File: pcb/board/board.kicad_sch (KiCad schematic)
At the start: 20 parts, among them J1 USB_C_Receptacle_USB2.0, J3 Micro_SD_Card_Det, J4 Conn_01x05_Male, J6 Conn_02x02_Top_Bottom

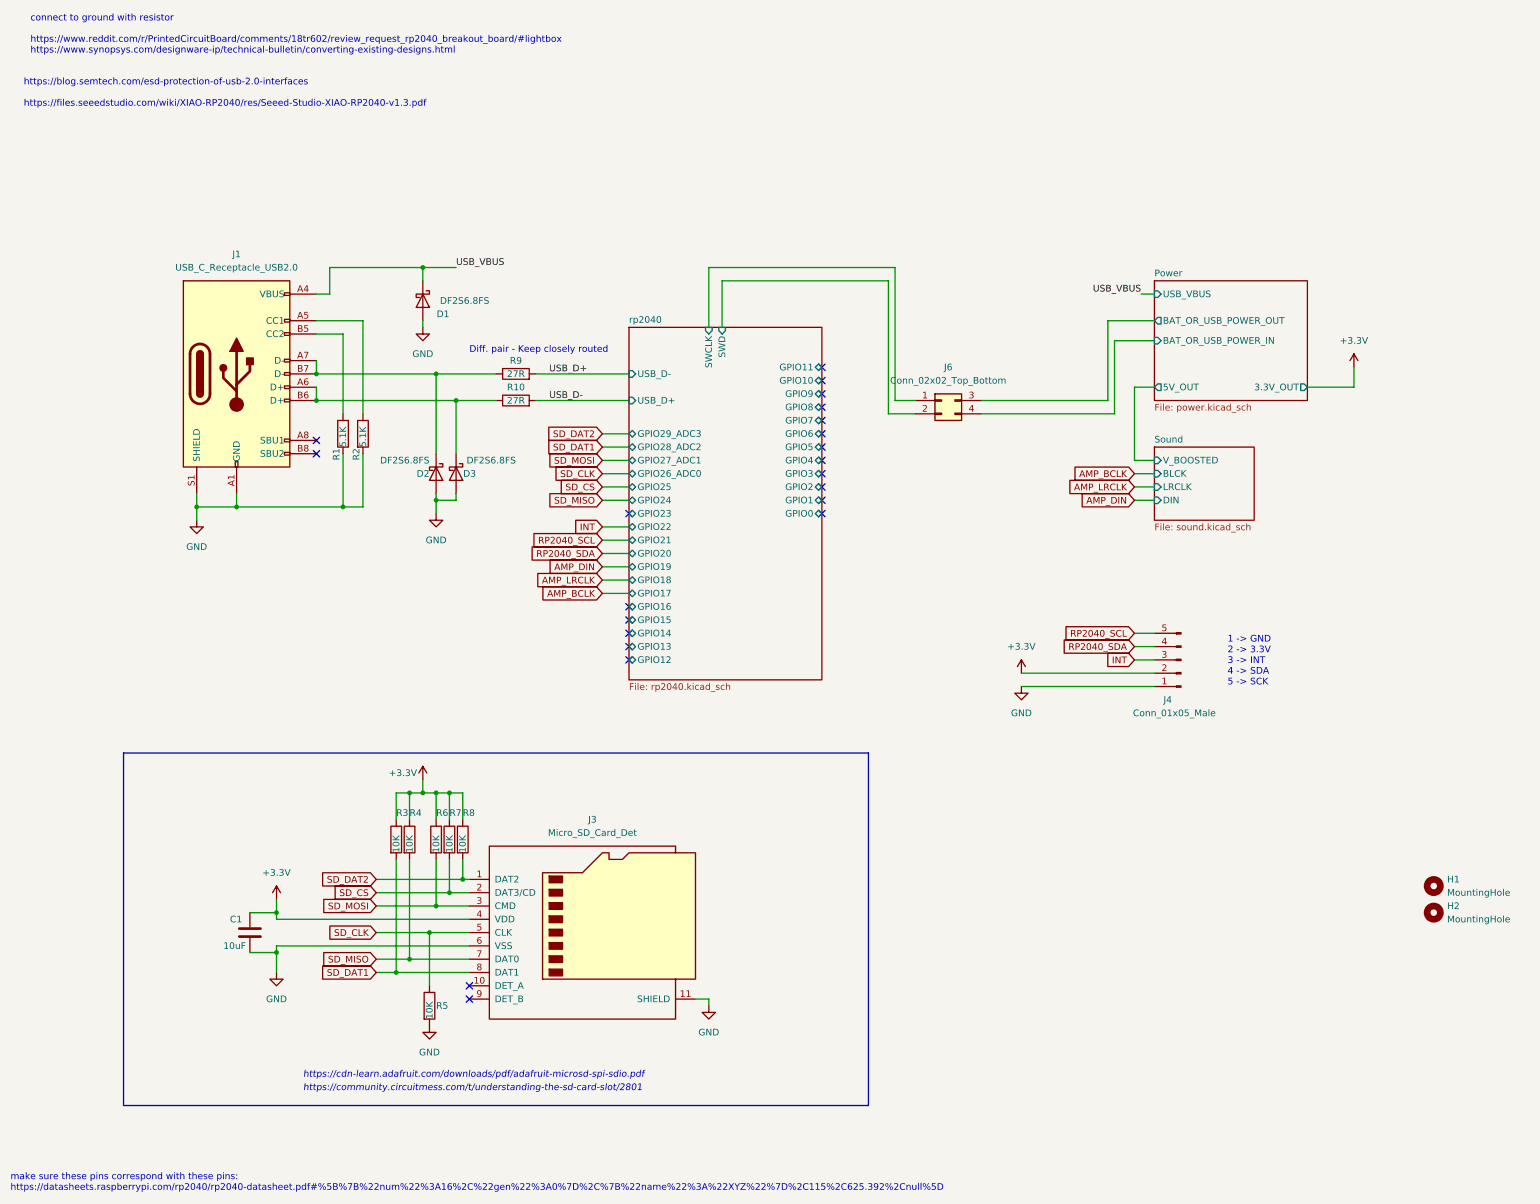
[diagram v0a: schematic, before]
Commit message: Update readme and pcb
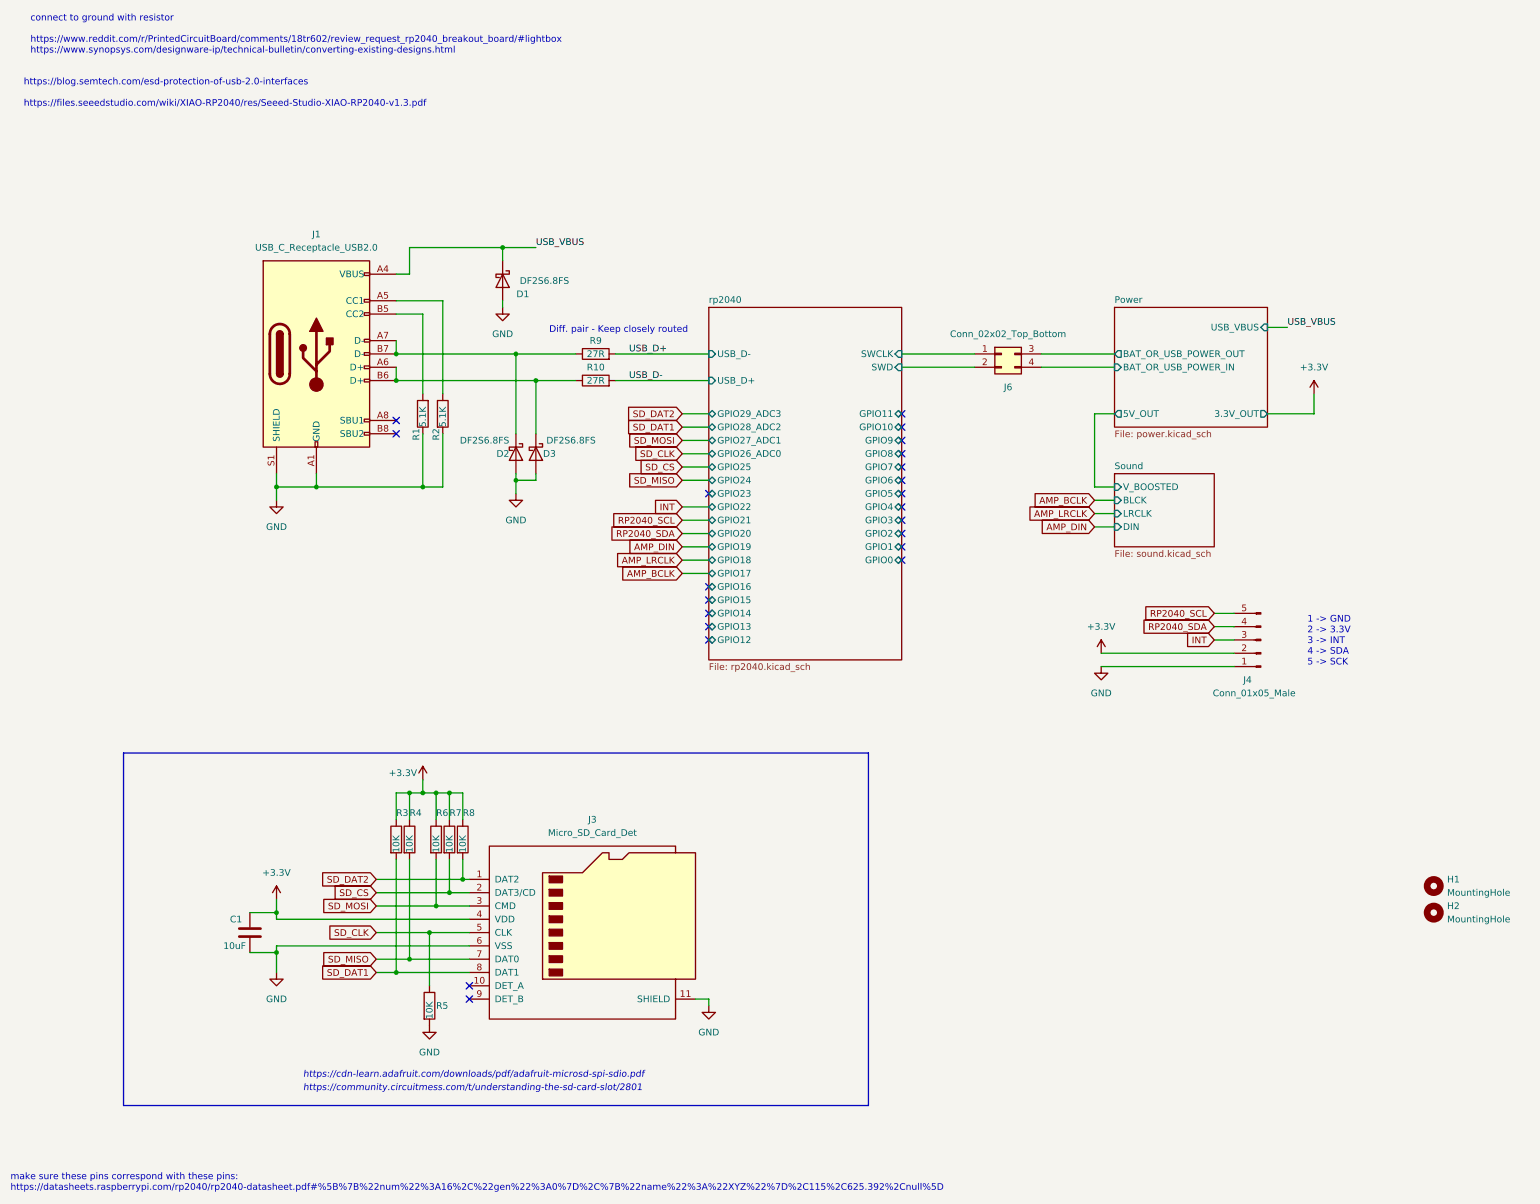
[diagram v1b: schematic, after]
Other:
- moved on the sheet: D1, D2, D3, J1, J4, J6, R1, R10, R2, R9
